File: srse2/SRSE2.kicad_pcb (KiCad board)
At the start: 2 copper layers, 82 x 72 mm, 93 parts, among them J1 s88-N, J2 CAN, P1 I2S, P10 PIC_SPARE, P11 RS485 TERM, P12 RS485, P13 CONN_01X03, P15 S88I, P17 RA5, P18 CONN_01X03, P19 CONN_01X02, P2 CONN_01X09, P20 O2P-Rst, P3 CONN_01X02, P4 CONN_01X04, P5 CONN_01X04, P6 ISO_I2C, P7 CAN_TERM, P8 CAN, P9 PIC_I2C, U1 Omega2, U10 OKI-78SR, U2 ADuM1250, U3 SN65HVD230, U4 PIC18F25K80, U5 HR911105A, U6 MAX485, U7 TPS5430DDA, U8 CD4504, U9 LM317, Y1 16MHz

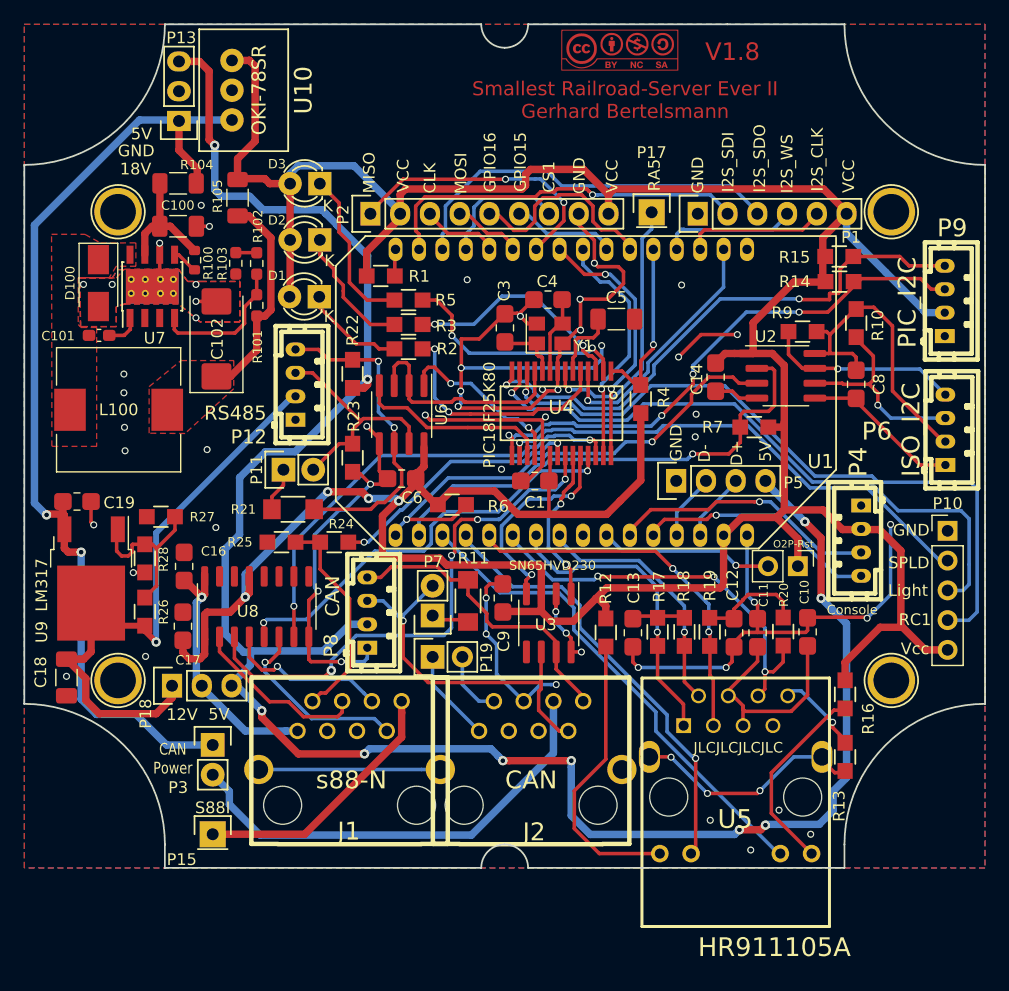
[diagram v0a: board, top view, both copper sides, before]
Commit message: add new production ZIP
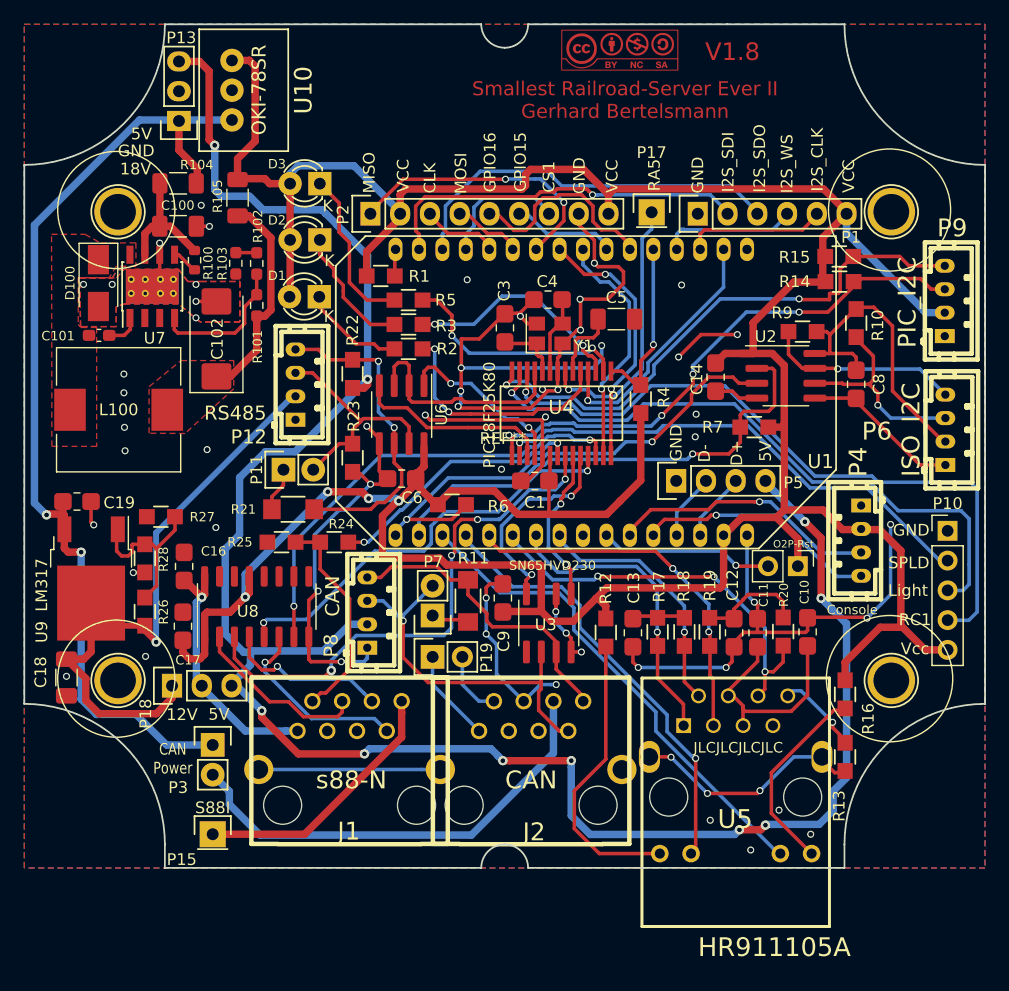
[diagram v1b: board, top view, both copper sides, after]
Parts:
- added REF**: Inlay, SRSE2:Inlay, F.Cu at (140.8, 109.8)
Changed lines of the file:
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@@
+    )
+  )
+  (footprint "SRSE2:Inlay" (layer "F.Cu")
+    (at 140.85 109.85)
+    (attr smd)
+    (fp_text reference "REF**" (at 0 -0.5 unlocked) (layer "F.SilkS")
+      (effects (font (size 1 1) (thickness 0.15)))
+    )
+    (fp_text value "Inlay" (at 0 1 unlocked) (layer "F.Fab")
+      (effects (font (size 1 1) (thickness 0.15)))
+    )
+    (fp_text user "${REFERENCE}" (at 0 2.5 unlocked) (layer "F.Fab")
+      (effects (font (size 1 1) (thickness 0.15)))
+    )
+    (fp_circle (center -33 20) (end -28 20) (layer "F.SilkS") (width 0.12) (fill none))
+    (fp_circle (center 33 -20) (end 38.211644 -20) (layer "F.SilkS") (width 0.12) (fill none))
+    (fp_circle (center 33 20) (end 38.391146 20) (layer "F.SilkS") (width 0.12) (fill none))
+    (fp_circle (center -33 -20) (end -28 -20) (layer "F.SilkS") (width 0.12) (fill none))
+    (fp_circle (center 33 20) (end 33.000001 20) (layer "F.SilkS") (width 0.12) (fill none))
+    (model "${KIPRJMOD}/inlay.wrl"
+      (offset (xyz 0 0 -4.6))
+      (scale (xyz 1 1 1))
+      (rotate (xyz 0 0 0))
     )
   )
